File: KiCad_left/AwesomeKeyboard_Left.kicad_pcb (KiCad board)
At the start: 2 copper layers, 140 x 109 mm, 57 parts, among them J1 AudioJack4_Ground, SW1 SW_DIP_x01, SW11 SW_Push, SW12 SW_Push, SW13 SW_Push, SW14 SW_Push, SW15 SW_Push, SW16 SW_Push, SW21 SW_Push, SW22 SW_Push, SW23 SW_Push, SW24 SW_Push, SW25 SW_Push, SW26 SW_Push, SW31 SW_Push, SW32 SW_Push, SW33 SW_Push, SW34 SW_Push, SW35 SW_Push, SW36 SW_Push, SW45 SW_Push, SW46 SW_Push

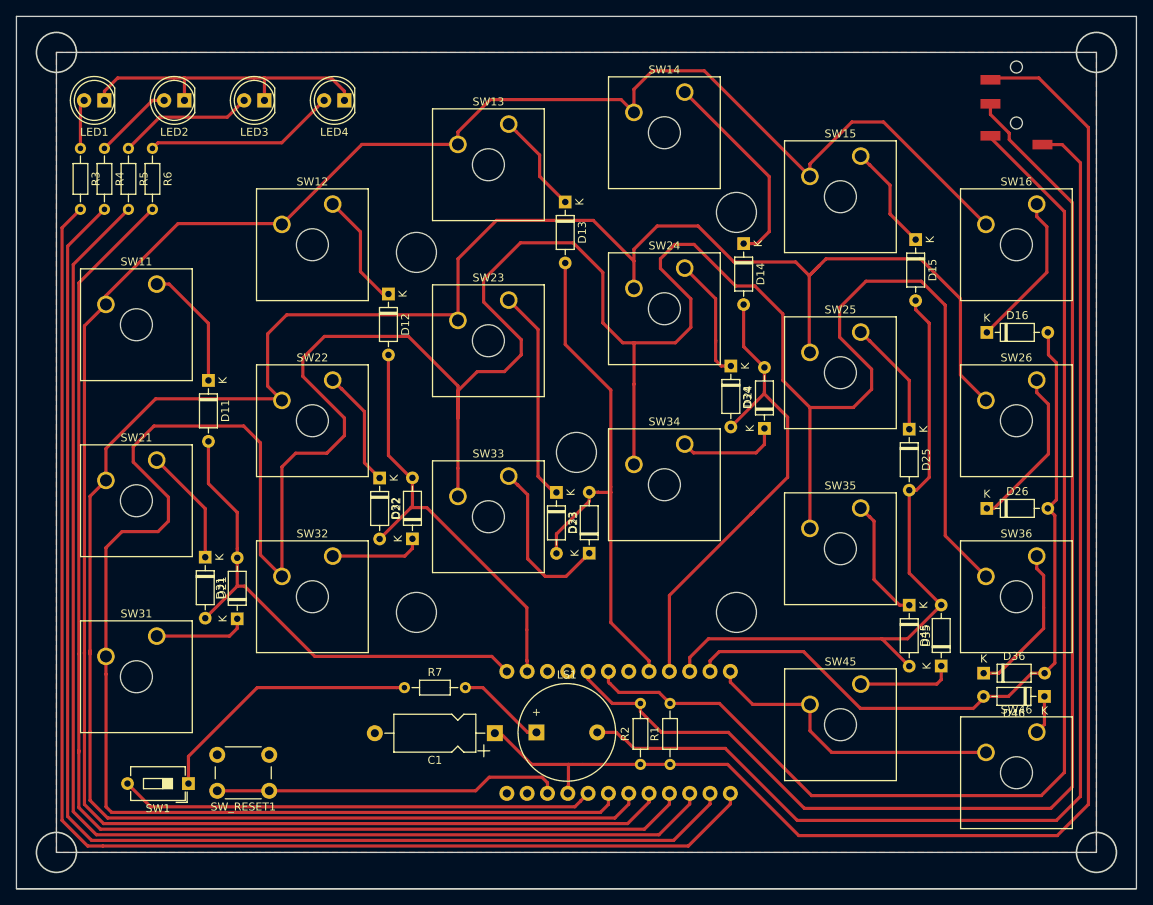
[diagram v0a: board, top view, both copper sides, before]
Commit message: restart
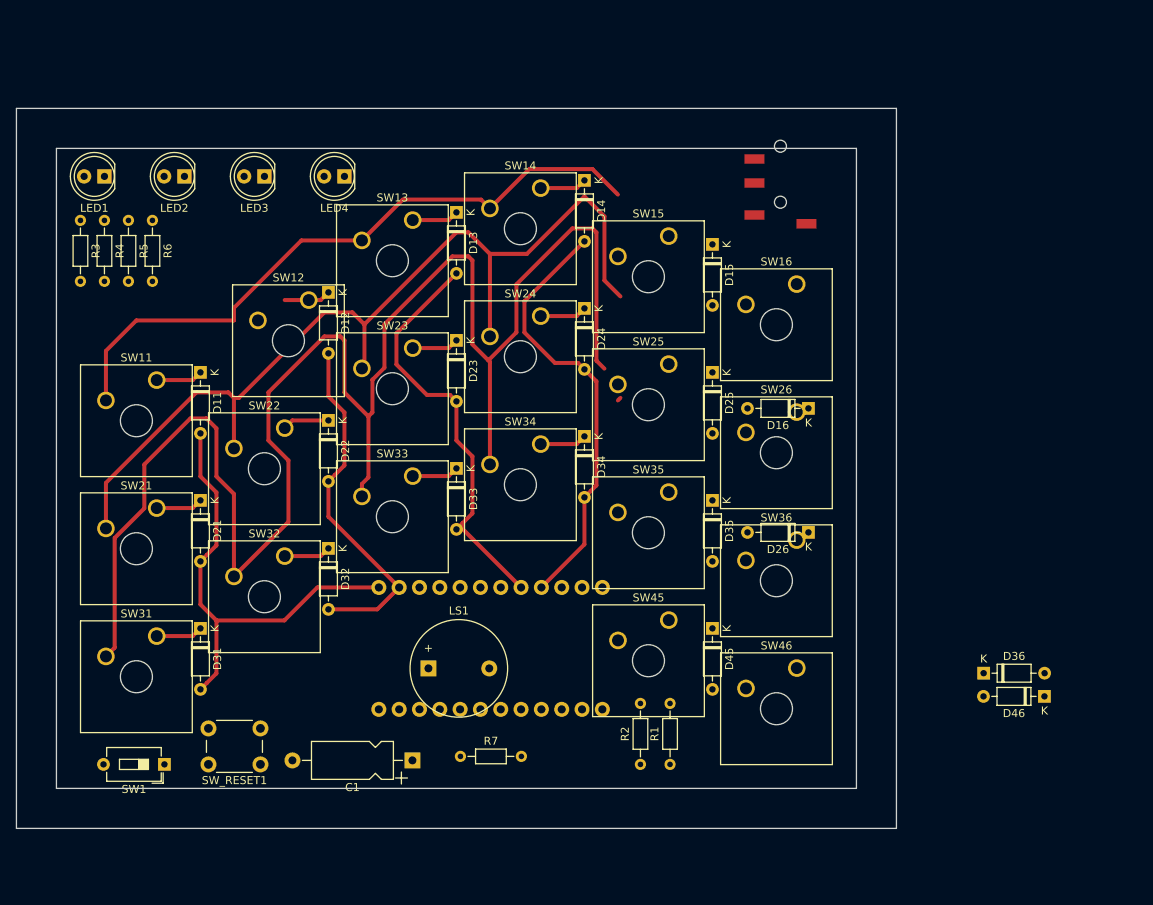
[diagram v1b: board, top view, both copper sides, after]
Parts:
- moved SW16 31.6 mm to (170.3, 103.6)
- moved J1 31.1 mm to (168.3, 91.2)
- moved SW46 31.0 mm to (170.3, 151.6)
- moved SW26 30.3 mm to (170.3, 119.6)
- moved SW36 30.1 mm to (170.3, 135.6)
- moved D45 29.0 mm to (159.8, 146.7), turned to 270 degrees
- moved D35 27.9 mm to (159.8, 130.7)
- moved SW15 26.0 mm to (154.3, 97.6)
- moved D25 25.6 mm to (159.8, 114.7)
- moved D15 25.4 mm to (159.8, 98.7)
- moved SW45 25.3 mm to (154.3, 145.6)
- moved SW25 24.3 mm to (154.3, 113.6)
- moved D16 24.2 mm to (171.8, 119.2), turned to 180 degrees
- moved SW35 24.1 mm to (154.3, 129.6)
- moved D23 22.7 mm to (127.8, 110.7)
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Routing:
- net /ROW3: track 432.7 -> 212.8 mm
- net /ROW1: track 278.8 -> 82.7 mm
- net GND: track 190.4 -> 0.00 mm
- net VCC: track 184.3 -> 0.00 mm
- net /LED1: track 165.7 -> 0.00 mm
- net /ROW2: track 285.7 -> 121.4 mm
- net /LED2: track 162.5 -> 0.00 mm
- net Net-(B1-Pad5): track 159.5 -> 0.00 mm
- net /LED3: track 159.3 -> 0.00 mm
- net /LED4: track 156.4 -> 0.00 mm
- net Net-(B1-Pad6): track 148.8 -> 0.00 mm
- net /COL6: track 92.6 -> 0.00 mm
- net /COL5: track 82.7 -> 0.00 mm
- net /SPEAKER: track 59.5 -> 0.00 mm
- net Net-(B1-Pad22): track 43.6 -> 0.00 mm
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- removed copper zone on F.Cu, net GND
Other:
- board size 140 x 109 mm -> 110 x 90 mm
- net class Default: trace_width 0.4 -> 0.5
